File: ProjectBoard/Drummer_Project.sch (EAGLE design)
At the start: 9 parts, among them J1 292303-1, SW1 PUSH_BUTTON, U1 POCKETBEAGLE, U2 SERVO_SG90, U3 SERVO_SG90

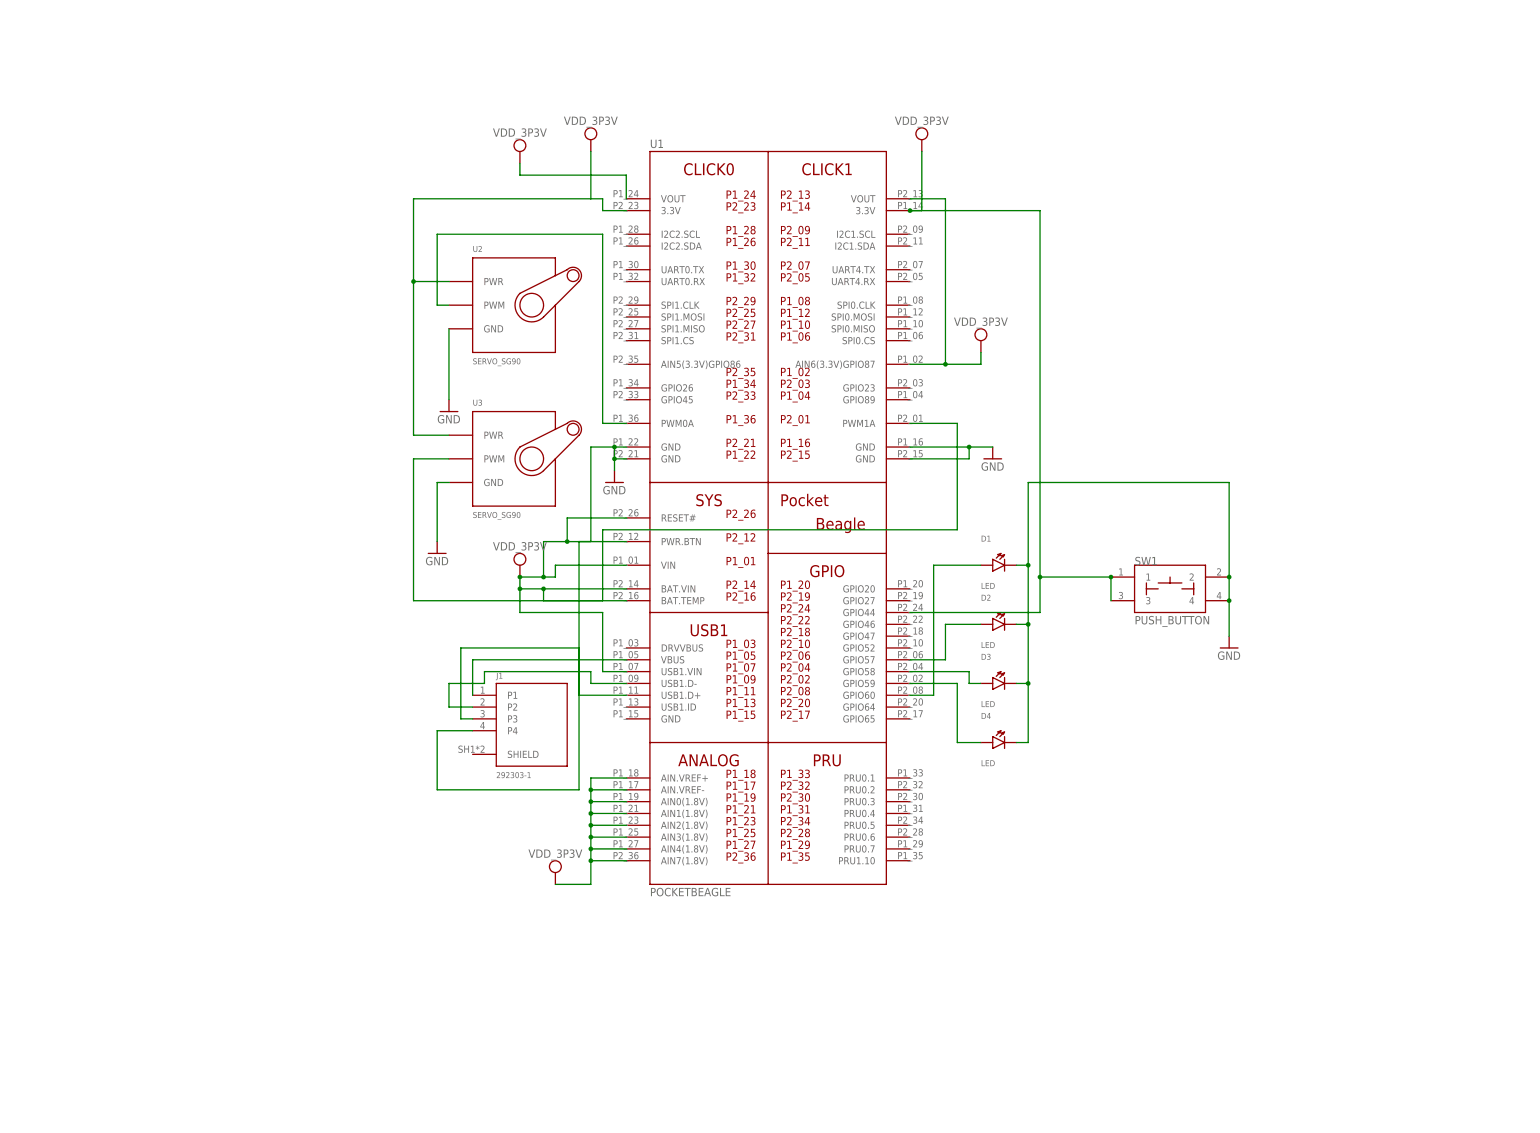
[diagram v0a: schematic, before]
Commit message: Changes!
here
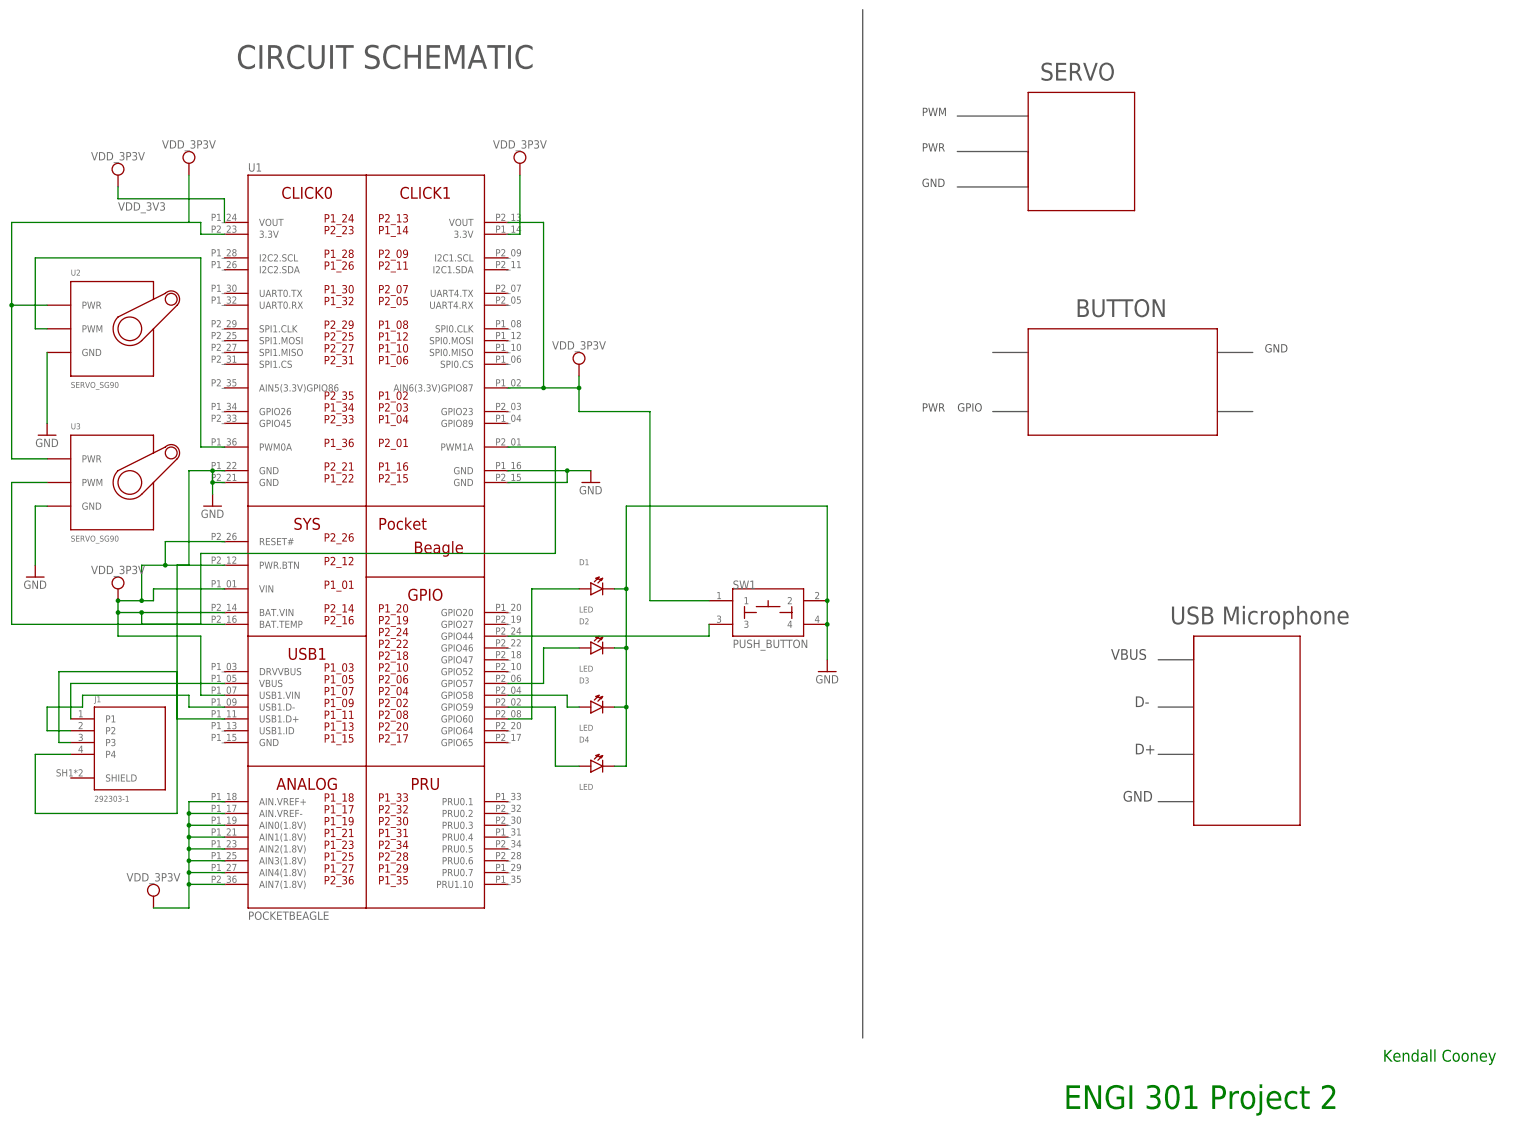
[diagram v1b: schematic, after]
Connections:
- removed net N$23: SW1.1, SW1.3, U1.3.3V@1, U1.3.3V@2, U1.AIN.VREF+, U1.AIN.VREF-, U1.AIN0(1.8V), U1.AIN1(1.8V), U1.AIN2(1.8V), U1.AIN3(1.8V), U1.AIN4(1.8V), U1.AIN6(3.3V)GPIO87, U1.AIN7(1.8V), U1.BAT.TEMP, U1.BAT.VIN, U1.GPIO44, U1.PWR.BTN, U1.RESET#, U1.USB1.VIN, U1.VIN, U1.VOUT@2, U2.PWR, U3.PWR
- removed net VDD_3P3V: U1.VOUT@1
- new net N$1: SW1.3, U1.GPIO44
- new net VDD_3V3: SW1.1, U1.3.3V@1, U1.3.3V@2, U1.AIN.VREF+, U1.AIN.VREF-, U1.AIN0(1.8V), U1.AIN1(1.8V), U1.AIN2(1.8V), U1.AIN3(1.8V), U1.AIN4(1.8V), U1.AIN6(3.3V)GPIO87, U1.AIN7(1.8V), U1.BAT.TEMP, U1.BAT.VIN, U1.PWR.BTN, U1.RESET#, U1.USB1.VIN, U1.VIN, U1.VOUT@1, U1.VOUT@2, U2.PWR, U3.PWR
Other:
- note added: "BUTTON"
- note added: "CIRCUIT SCHEMATIC"
- note added: "D+"
- note added: "D-"
- note added: "ENGI 301 Project 2"
- note added: "GND"
- note added: "GPIO"
- note added: "Kendall Cooney"
- note added: "PWM"
- note added: "PWR"
- note added: "SERVO"
- note added: "USB Microphone"
- note added: "VBUS"
- moved on the sheet: D1, D2, D3, D4, J1, SW1, U1, U2, U3
